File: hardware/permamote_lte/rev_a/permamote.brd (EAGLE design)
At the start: 27 x 60 mm, 117 parts, among them IC1 NRF9160, J1 TC2030-JLINK-NL, J2 U.FL-R-SMT, J3 NANO_SIM, J4 U.FL-R-SMT, J5 DM3AT-SF-PEJM5, Q1 PMDXB950UPEL, Q10 PMDXB950UPEL, Q2 PMDXB950UPEL, Q3 PMDXB950UPEL, Q4 PMDXB950UPEL, Q5 PMDXB950UPEL, Q6 PMDXB950UPEL, Q7 PMDXB950UPEL, Q8 PMDXB950UPEL, U1 AB1815-T3, U10 SIP32510, U11 SI7021-A20-GM1, U12 TCS34725, U2 BQ25505, U3 EKMB1101111, U4 BGA725L6, U5 TPD3F303DPVR, U6 LIS2DW12, U7 MAX17222, U8 MAX44009, U9 MS5637-02BA03, X4 ABS07-32.768KHZ-7-T

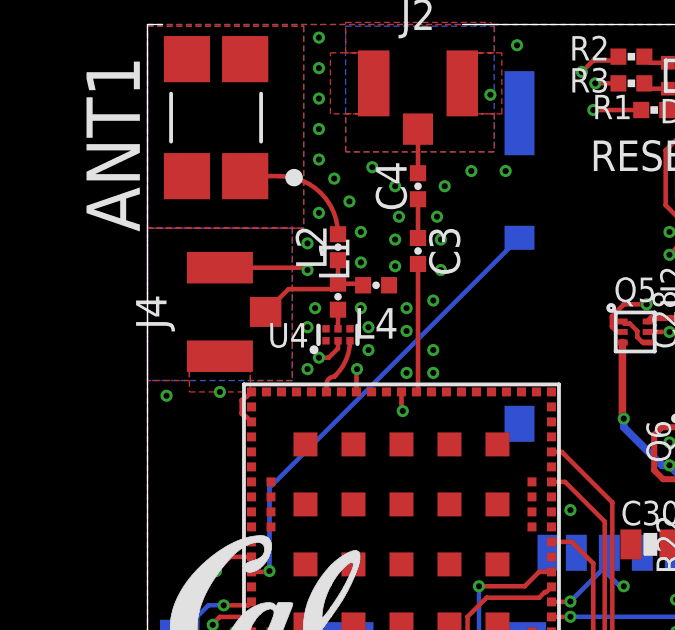
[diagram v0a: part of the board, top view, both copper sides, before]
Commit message: more routing fixes
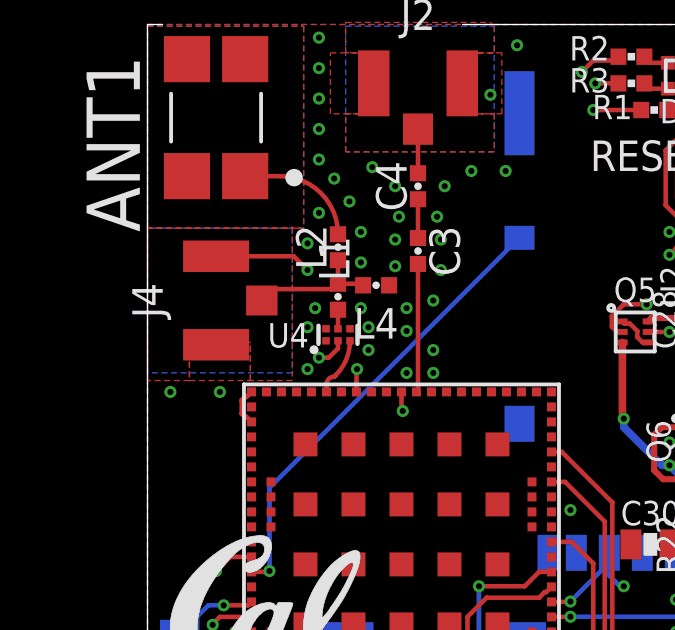
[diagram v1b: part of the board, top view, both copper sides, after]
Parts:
- moved J4 0.40 mm to (2.29, 50.8)
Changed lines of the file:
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@@
 <attribute name="NAME" x="6.731" y="52.197" size="1.016" layer="25" font="vector" ratio="12" rot="R90" align="bottom-center"/>
 </element>
-<element name="J4" library="connector" package="U.FL_SMT" value="U.FL-R-SMT" x="2.413" y="50.419" smashed="yes" rot="R90">
-<attribute name="DIGIKEY" value="H122041-ND" x="2.413" y="50.419" size="1.778" layer="27" rot="R90" display="off"/>
-<attribute name="MANUFACTURER" value="Hirose" x="2.413" y="50.419" size="1.778" layer="27" rot="R90" display="off"/>
-<attribute name="MPN" value="U.FL-R-SMT-1(01)" x="2.413" y="50.419" size="1.778" layer="27" rot="R90" display="off"/>
-<attribute name="NAME" x="-0.381" y="50.419" size="1.016" layer="25" font="vector" ratio="12" rot="R270" align="bottom-center"/>
+<element name="J4" library="connector" package="U.FL_SMT" value="U.FL-R-SMT" x="2.286" y="50.8" smashed="yes" rot="R90">
+<attribute name="DIGIKEY" value="H122041-ND" x="2.286" y="50.8" size="1.778" layer="27" rot="R90" display="off"/>
+<attribute name="MANUFACTURER" value="Hirose" x="2.286" y="50.8" size="1.778" layer="27" rot="R90" display="off"/>
+<attribute name="MPN" value="U.FL-R-SMT-1(01)" x="2.286" y="50.8" size="1.778" layer="27" rot="R90" display="off"/>
+<attribute name="NAME" x="-0.508" y="50.8" size="1.016" layer="25" font="vector" ratio="12" rot="R270" align="bottom-center"/>
 </element>
 <element name="ANT1" library="1462350001" package="ANT_1462350001" value="1462350001" x="2.286" y="56.896" smashed="yes" rot="R90">
@@
 <wire x1="6.966" y1="48.495" x2="6.985" y2="48.514" width="0.1524" layer="1" curve="-90"/>
 <wire x1="12.396" y1="57.041" x2="12.192" y2="57.245" width="0.1524" layer="16"/>
-<via x="0.635" y="47.625" extent="1-16" drill="0.2032"/>
+<via x="0.762" y="47.752" extent="1-16" drill="0.2032"/>
 <via x="5.334" y="48.514" extent="1-16" drill="0.2032"/>
 <via x="5.334" y="52.705" extent="1-16" drill="0.2032"/>
@@
 <polygon width="0.1524" layer="1">
 <vertex x="1.397" y="49.403"/>
-<vertex x="1.397" y="47.752"/>
-<vertex x="3.429" y="47.752"/>
+<vertex x="1.397" y="48.133"/>
+<vertex x="3.429" y="48.133"/>
 <vertex x="3.429" y="49.403"/>
 </polygon>
@@
 <via x="11.938" y="55.118" extent="1-16" drill="0.2032"/>
 <via x="12.319" y="59.309" extent="1-16" drill="0.2032"/>
-<wire x1="2.413" y1="51.894" x2="5.256" y2="51.894" width="0.1524" layer="1"/>
-<wire x1="5.256" y1="51.894" x2="5.334" y2="51.816" width="0.1524" layer="1"/>
+<wire x1="2.286" y1="52.275" x2="4.875" y2="52.275" width="0.1524" layer="1"/>
+<wire x1="4.875" y1="52.275" x2="5.334" y2="51.816" width="0.1524" layer="1"/>
 </signal>
 <signal name="VCC">
@@
 <wire x1="6.35" y1="52.14493125" x2="6.35" y2="51.36006875" width="0.1524" layer="1"/>
 <wire x1="6.35" y1="51.36006875" x2="6.126515625" y2="51.181" width="0.1524" layer="1"/>
-<wire x1="6.126515625" y1="51.181" x2="4.7" y2="51.181" width="0.1524" layer="1"/>
-<wire x1="4.7" y1="51.181" x2="3.938" y2="50.419" width="0.1524" layer="1"/>
+<wire x1="6.126515625" y1="51.181" x2="4.192" y2="51.181" width="0.1524" layer="1"/>
+<wire x1="4.192" y1="51.181" x2="3.811" y2="50.8" width="0.1524" layer="1"/>
 <wire x1="6.35" y1="51.36006875" x2="7.200503125" y2="51.36006875" width="0.1524" layer="1"/>
 <wire x1="7.18693125" y1="51.308" x2="7.200503125" y2="51.36006875" width="0.1524" layer="1"/>
@@
 <signal name="N$39">
 <polygon width="0.1524" layer="2" pour="cutout">
-<vertex x="4.826" y="48.133"/>
-<vertex x="0" y="48.133"/>
+<vertex x="4.826" y="48.387"/>
+<vertex x="0" y="48.387"/>
 <vertex x="0" y="53.213"/>
 <vertex x="4.826" y="53.213"/>
@@
 <signal name="N$43">
 <polygon width="0.1524" layer="15" pour="cutout">
-<vertex x="4.826" y="48.133"/>
-<vertex x="0" y="48.133"/>
+<vertex x="4.826" y="48.387"/>
+<vertex x="0" y="48.387"/>
 <vertex x="0" y="53.213"/>
 <vertex x="4.826" y="53.213"/>
@@
 <polygon width="0.1524" layer="16" pour="cutout">
 <vertex x="4.826" y="53.213"/>
-<vertex x="4.826" y="48.133"/>
-<vertex x="0" y="48.133"/>
+<vertex x="4.826" y="48.387"/>
+<vertex x="0" y="48.387"/>
 <vertex x="0" y="53.213"/>
 </polygon>
